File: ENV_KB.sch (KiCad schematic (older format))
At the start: 180 parts, among them J1 USB_C_Receptacle

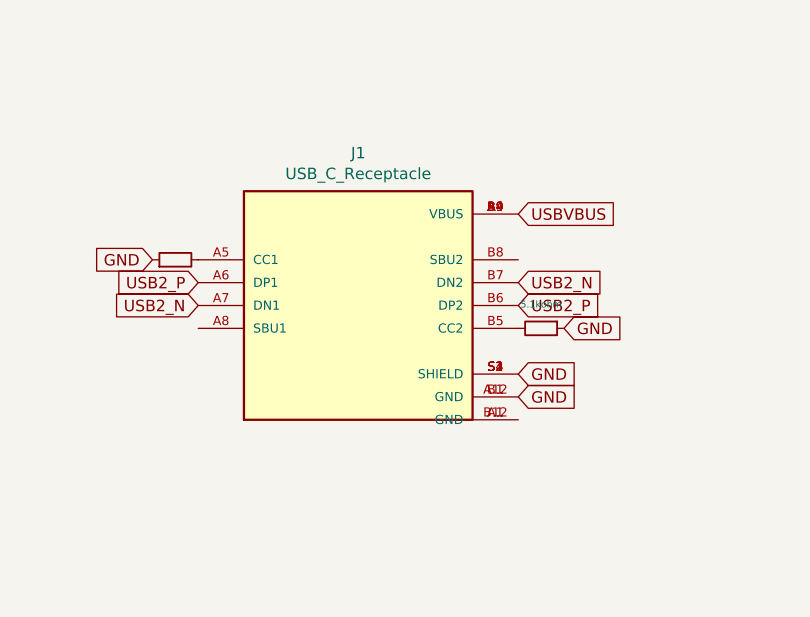
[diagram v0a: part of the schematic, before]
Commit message: some adjustments
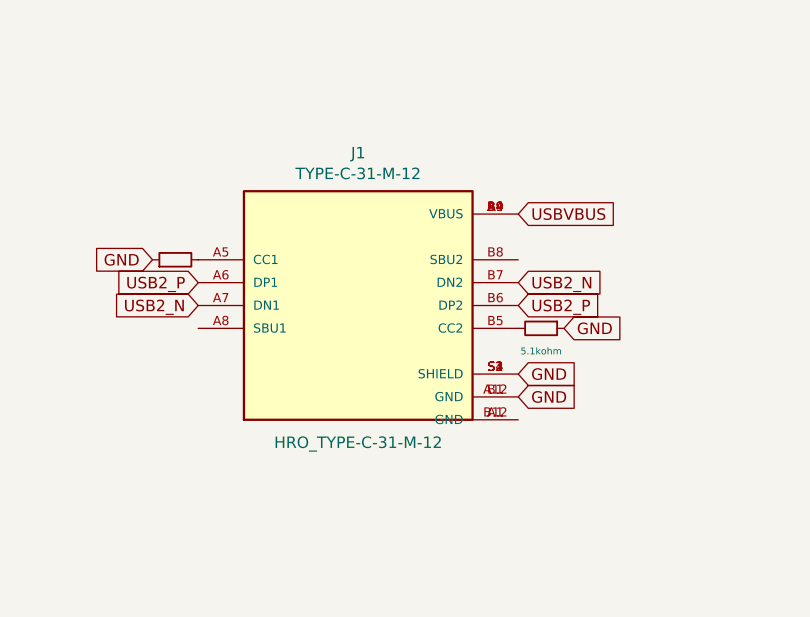
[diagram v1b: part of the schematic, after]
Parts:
- J1: value USB_C_Receptacle -> TYPE-C-31-M-12; footprint Type-C-Bits:HRO_TYPE-C-31-M-12 -> HRO_TYPE-C-31-M-12; MANUFACTURER (none) -> HRO Electronics; MAXIMUM_PACKAGE_HEIGHT (none) -> 3.31mm; PARTREV (none) -> A; STANDARD (none) -> Manufacturer Recommendations
- RPI1: footprint MCU_RaspberryPi_and_Boards.pretty:RPi_Pico_SMD_TH -> EM_Extras:RPi_Pico_SMD_TH
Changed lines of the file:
@@
 F 0 "RPI1" H 13000 10550 50  0000 C CNN
 F 1 "Pico" H 12800 10550 50  0000 C CNN
-F 2 "MCU_RaspberryPi_and_Boards.pretty:RPi_Pico_SMD_TH" V 12950 10050 50  0001 C CNN
+F 2 "EM_Extras:RPi_Pico_SMD_TH" V 12950 10050 50  0001 C CNN
 F 3 "" H 12950 10050 50  0001 C CNN
 	1    12950 10050
@@
 P 9950 8950
 F 0 "RESISTOR1" V 9754 8950 39  0001 C CNN
-F 1 "5.1kohm" V 9845 8950 30  0000 C CNN
+F 1 "5.1kohm" V 10050 8950 30  0000 C CNN
 F 2 "Resistor_SMD:R_0402_1005Metric" H 9950 8950 50  0001 C CNN
 F 3 "~" H 9950 8950 50  0001 C CNN
@@
 P 9150 8850
 F 0 "J1" H 9150 9517 50  0000 C CNN
-F 1 "USB_C_Receptacle" H 9150 9426 50  0000 C CNN
-F 2 "Type-C-Bits:HRO_TYPE-C-31-M-12" H 9300 8850 50  0001 C CNN
-F 3 "https://www.usb.org/sites/default/files/documents/usb_type-c.zip" H 9300 8850 50  0001 C CNN
+F 1 "TYPE-C-31-M-12" H 9150 9426 50  0000 C CNN
+F 2 "HRO_TYPE-C-31-M-12" H 9150 8250 50  0000 C CNN
+F 3 "~" H 9300 8850 50  0001 C CNN
+F 4 "HRO Electronics" H 9150 8850 50  0001 C CNN "MANUFACTURER"
+F 5 "3.31mm" H 9150 8850 50  0001 C CNN "MAXIMUM_PACKAGE_HEIGHT"
+F 6 "A" H 9150 8850 50  0001 C CNN "PARTREV"
+F 7 "Manufacturer Recommendations" H 9150 8850 50  0001 C CNN "STANDARD"
 	1    9150 8850
 	1    0    0    -1
